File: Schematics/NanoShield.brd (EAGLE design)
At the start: 17.8 x 43.2 mm, 20 parts, among them J1 HEAD15-NOSS, J2 HEAD15-NOSS-1, T1 , T2 

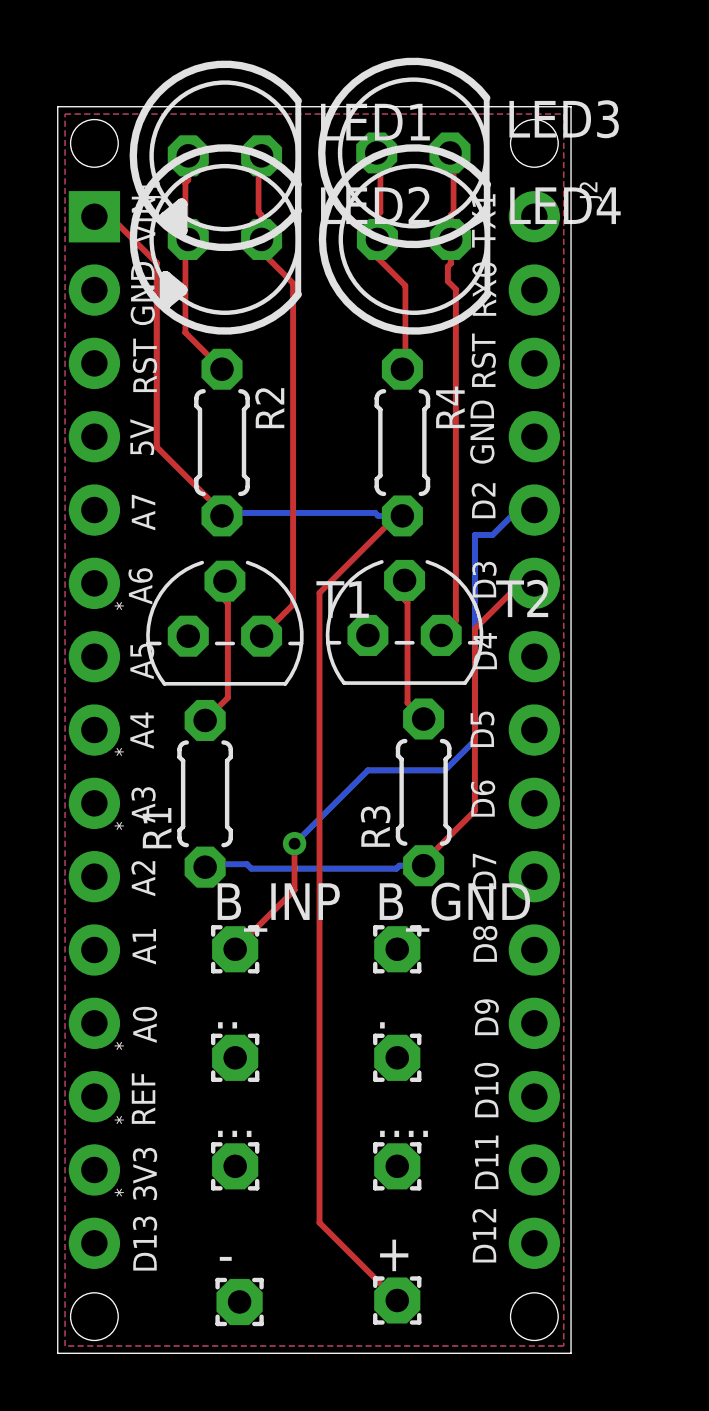
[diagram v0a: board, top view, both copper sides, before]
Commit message: Redesign
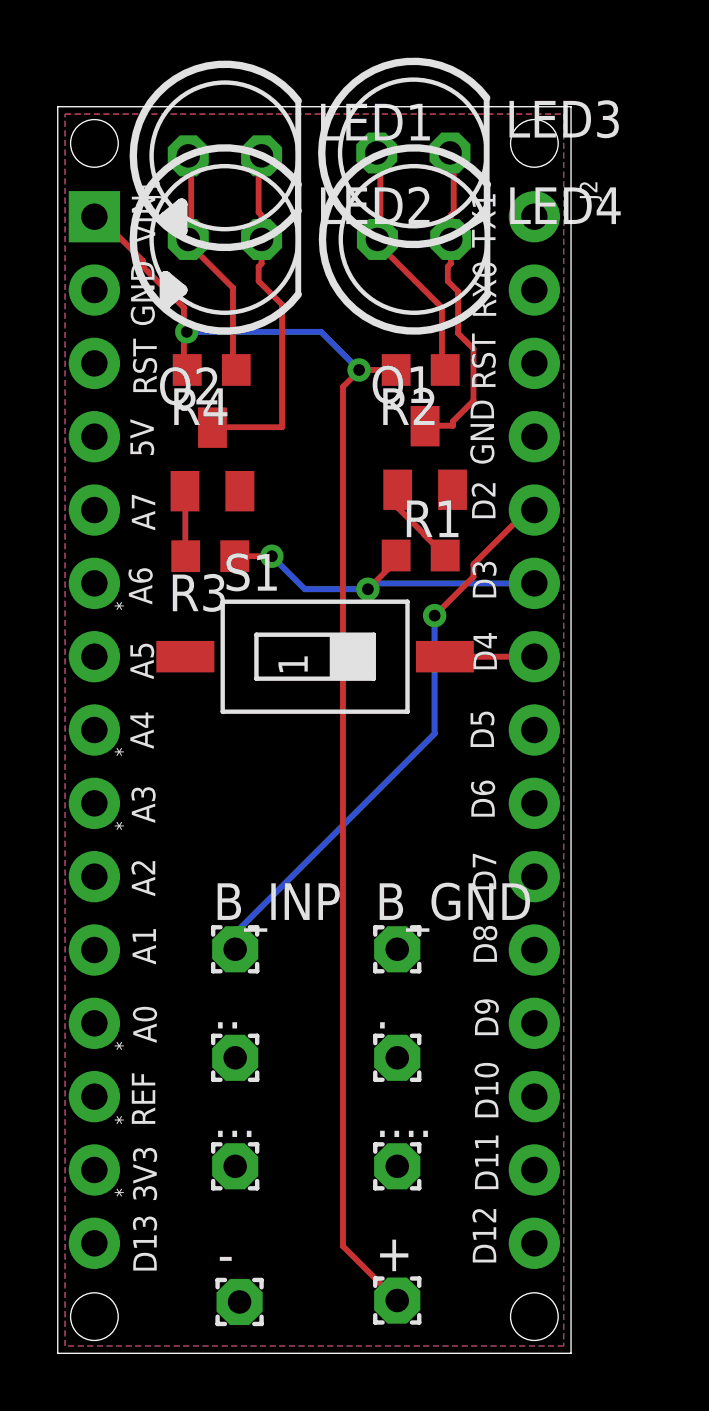
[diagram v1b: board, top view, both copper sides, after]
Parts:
- removed T1, T2: (no value), transistor:TO92
- added Q1, Q2: BCF81SMD, transistor-npn:SOT23-BEC
- added S1: SWS001, smd-special:SMS-001
- R1, R2, R3, R4: device resistor:0204/5 -> eagle-ltspice:R0603
- moved R1 11.1 mm to (12.6, 27.6), turned to 0 degrees
- moved R3 11.0 mm to (5.28, 27.6), turned to 180 degrees
- moved R2 7.33 mm to (12.6, 34.1), turned to 180 degrees
- moved R4 7.07 mm to (5.33, 34.1), turned to 180 degrees
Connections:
- new net N$1: J2.7, S1.2
- net COM: now also ...1, Q1.E, Q2.E, S1.1; no longer B_GND.1, J2.7, T1.3, T2.3
- net N$3: now also Q2.C; no longer T1.1
- net N$4: now also Q1.C; no longer T2.1
- net N$5: now also Q2.B, R3.2; no longer R1.2, T1.2
- net N$6: now also Q1.B, R1.2; no longer R3.2, T2.2
- net N$7: now also R4.1; no longer R2.1
- net N$8: now also R2.1; no longer R4.1
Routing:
- net N$9: track 19.5 -> 12.5 mm, vias 0 -> 2
- net N$4: track 17.2 -> 11.2 mm
- net N$3: track 17.6 -> 12.3 mm
- net N$1: track 0.00 -> 3.10 mm
- net N$5: track 5.19 -> 2.27 mm
- net N$6: track 5.07 -> 2.97 mm
- net N$10: track 21.8 -> 19.7 mm
- net VIN: track 49.7 -> 47.9 mm, vias 0 -> 2
- net N$8: track 8.03 -> 8.80 mm
